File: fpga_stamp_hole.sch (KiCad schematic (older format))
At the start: 0 parts

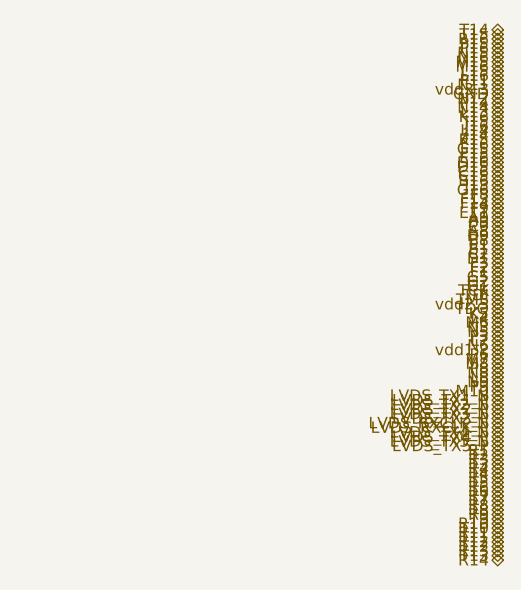
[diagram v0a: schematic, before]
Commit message: first commit
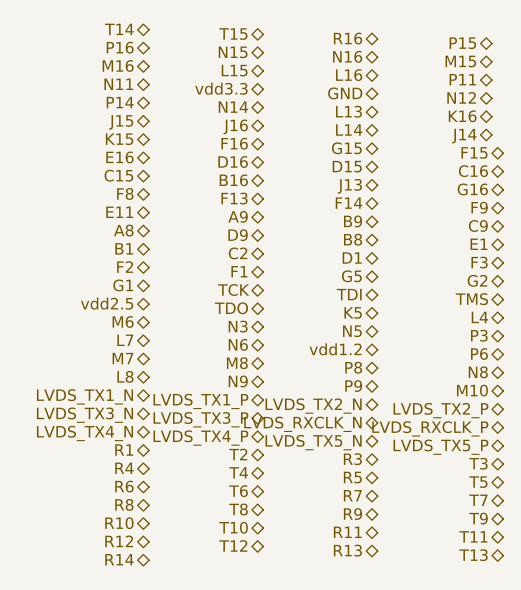
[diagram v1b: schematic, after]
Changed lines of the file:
@@
 $Descr A4 11693 8268
 encoding utf-8
-Sheet 2 2
+Sheet 2 3
 Title ""
 Date ""
@@
 EndData
 $EndBitmap
-Text HLabel 2550 1200 0    50   BiDi ~ 0
+Text HLabel 1000 1200 0    50   BiDi ~ 0
 T14
-Text HLabel 2550 1220 0    50   BiDi ~ 0
+Text HLabel 1500 1220 0    50   BiDi ~ 0
 T15
-Text HLabel 2550 1240 0    50   BiDi ~ 0
+Text HLabel 2000 1240 0    50   BiDi ~ 0
 R16
-Text HLabel 2550 1260 0    50   BiDi ~ 0
+Text HLabel 2500 1260 0    50   BiDi ~ 0
 P15
-Text HLabel 2550 1280 0    50   BiDi ~ 0
+Text HLabel 1000 1280 0    50   BiDi ~ 0
 P16
-Text HLabel 2550 1300 0    50   BiDi ~ 0
+Text HLabel 1500 1300 0    50   BiDi ~ 0
 N15
-Text HLabel 2550 1320 0    50   BiDi ~ 0
+Text HLabel 2000 1320 0    50   BiDi ~ 0
 N16
-Text HLabel 2550 1340 0    50   BiDi ~ 0
+Text HLabel 2500 1340 0    50   BiDi ~ 0
 M15
-Text HLabel 2550 1360 0    50   BiDi ~ 0
+Text HLabel 1000 1360 0    50   BiDi ~ 0
 M16
-Text HLabel 2550 1380 0    50   BiDi ~ 0
+Text HLabel 1500 1380 0    50   BiDi ~ 0
 L15
-Text HLabel 2550 1400 0    50   BiDi ~ 0
+Text HLabel 2000 1400 0    50   BiDi ~ 0
 L16
-Text HLabel 2550 1420 0    50   BiDi ~ 0
+Text HLabel 2500 1420 0    50   BiDi ~ 0
 P11
-Text HLabel 2550 1440 0    50   BiDi ~ 0
+Text HLabel 1000 1440 0    50   BiDi ~ 0
 N11
-Text HLabel 2550 1460 0    50   BiDi ~ 0
+Text HLabel 1500 1460 0    50   BiDi ~ 0
 vdd3.3
-Text HLabel 2550 1480 0    50   BiDi ~ 0
+Text HLabel 2000 1480 0    50   BiDi ~ 0
 GND
-Text HLabel 2550 1500 0    50   BiDi ~ 0
+Text HLabel 2500 1500 0    50   BiDi ~ 0
 N12
-Text HLabel 2550 1520 0    50   BiDi ~ 0
+Text HLabel 1000 1520 0    50   BiDi ~ 0
 P14
-Text HLabel 2550 1540 0    50   BiDi ~ 0
+Text HLabel 1500 1540 0    50   BiDi ~ 0
 N14
-Text HLabel 2550 1560 0    50   BiDi ~ 0
+Text HLabel 2000 1560 0    50   BiDi ~ 0
 L13
-Text HLabel 2550 1580 0    50   BiDi ~ 0
+Text HLabel 2500 1580 0    50   BiDi ~ 0
 K16
-Text HLabel 2550 1600 0    50   BiDi ~ 0
+Text HLabel 1000 1600 0    50   BiDi ~ 0
 J15
-Text HLabel 2550 1620 0    50   BiDi ~ 0
+Text HLabel 1500 1620 0    50   BiDi ~ 0
 J16
-Text HLabel 2550 1640 0    50   BiDi ~ 0
+Text HLabel 2000 1640 0    50   BiDi ~ 0
 L14
-Text HLabel 2550 1660 0    50   BiDi ~ 0
+Text HLabel 2500 1660 0    50   BiDi ~ 0
 J14
-Text HLabel 2550 1680 0    50   BiDi ~ 0
+Text HLabel 1000 1680 0    50   BiDi ~ 0
 K15
-Text HLabel 2550 1700 0    50   BiDi ~ 0
+Text HLabel 1500 1700 0    50   BiDi ~ 0
 F16
-Text HLabel 2550 1720 0    50   BiDi ~ 0
+Text HLabel 2000 1720 0    50   BiDi ~ 0
 G15
 Text HLabel 2550 1740 0    50   BiDi ~ 0
 F15
-Text HLabel 2550 1760 0    50   BiDi ~ 0
+Text HLabel 1000 1760 0    50   BiDi ~ 0
 E16
-Text HLabel 2550 1780 0    50   BiDi ~ 0
+Text HLabel 1500 1780 0    50   BiDi ~ 0
 D16
-Text HLabel 2550 1800 0    50   BiDi ~ 0
+Text HLabel 2000 1800 0    50   BiDi ~ 0
 D15
 Text HLabel 2550 1820 0    50   BiDi ~ 0
 C16
-Text HLabel 2550 1840 0    50   BiDi ~ 0
+Text HLabel 1000 1840 0    50   BiDi ~ 0
 C15
-Text HLabel 2550 1860 0    50   BiDi ~ 0
+Text HLabel 1500 1860 0    50   BiDi ~ 0
 B16
-Text HLabel 2550 1880 0    50   BiDi ~ 0
+Text HLabel 2000 1880 0    50   BiDi ~ 0
 J13
 Text HLabel 2550 1900 0    50   BiDi ~ 0
 G16
-Text HLabel 2550 1920 0    50   BiDi ~ 0
+Text HLabel 1000 1920 0    50   BiDi ~ 0
 F8
-Text HLabel 2550 1940 0    50   BiDi ~ 0
+Text HLabel 1500 1940 0    50   BiDi ~ 0
 F13
-Text HLabel 2550 1960 0    50   BiDi ~ 0
+Text HLabel 2000 1960 0    50   BiDi ~ 0
 F14
 Text HLabel 2550 1980 0    50   BiDi ~ 0
 F9
-Text HLabel 2550 2000 0    50   BiDi ~ 0
+Text HLabel 1000 2000 0    50   BiDi ~ 0
 E11
-Text HLabel 2550 2020 0    50   BiDi ~ 0
+Text HLabel 1500 2020 0    50   BiDi ~ 0
 A9
-Text HLabel 2550 2040 0    50   BiDi ~ 0
+Text HLabel 2000 2040 0    50   BiDi ~ 0
 B9
 Text HLabel 2550 2060 0    50   BiDi ~ 0
 C9
-Text HLabel 2550 2080 0    50   BiDi ~ 0
+Text HLabel 1000 2080 0    50   BiDi ~ 0
 A8
-Text HLabel 2550 2100 0    50   BiDi ~ 0
+Text HLabel 1500 2100 0    50   BiDi ~ 0
 D9
-Text HLabel 2550 2120 0    50   BiDi ~ 0
+Text HLabel 2000 2120 0    50   BiDi ~ 0
 B8
 Text HLabel 2550 2140 0    50   BiDi ~ 0
 E1
-Text HLabel 2550 2160 0    50   BiDi ~ 0
+Text HLabel 1000 2160 0    50   BiDi ~ 0
 B1
-Text HLabel 2550 2180 0    50   BiDi ~ 0
+Text HLabel 1500 2180 0    50   BiDi ~ 0
 C2
-Text HLabel 2550 2200 0    50   BiDi ~ 0
+Text HLabel 2000 2200 0    50   BiDi ~ 0
 D1
 Text HLabel 2550 2220 0    50   BiDi ~ 0
 F3
-Text HLabel 2550 2240 0    50   BiDi ~ 0
+Text HLabel 1000 2240 0    50   BiDi ~ 0
 F2
-Text HLabel 2550 2260 0    50   BiDi ~ 0
+Text HLabel 1500 2260 0    50   BiDi ~ 0
 F1
-Text HLabel 2550 2280 0    50   BiDi ~ 0
+Text HLabel 2000 2280 0    50   BiDi ~ 0
 G5
 Text HLabel 2550 2300 0    50   BiDi ~ 0
 G2
-Text HLabel 2550 2320 0    50   BiDi ~ 0
+Text HLabel 1000 2320 0    50   BiDi ~ 0
 G1
-Text HLabel 2550 2340 0    50   BiDi ~ 0
+Text HLabel 1500 2340 0    50   BiDi ~ 0
 TCK
-Text HLabel 2550 2360 0    50   BiDi ~ 0
+Text HLabel 2000 2360 0    50   BiDi ~ 0
 TDI
 Text HLabel 2550 2380 0    50   BiDi ~ 0
 TMS
-Text HLabel 2550 2400 0    50   BiDi ~ 0
+Text HLabel 1000 2400 0    50   BiDi ~ 0
 vdd2.5
-Text HLabel 2550 2420 0    50   BiDi ~ 0
+Text HLabel 1500 2420 0    50   BiDi ~ 0
 TDO
-Text HLabel 2550 2440 0    50   BiDi ~ 0
+Text HLabel 2000 2440 0    50   BiDi ~ 0
 K5
 Text HLabel 2550 2460 0    50   BiDi ~ 0
 L4
-Text HLabel 2550 2480 0    50   BiDi ~ 0
+Text HLabel 1000 2480 0    50   BiDi ~ 0
 M6
-Text HLabel 2550 2500 0    50   BiDi ~ 0
+Text HLabel 1500 2500 0    50   BiDi ~ 0
 N3
-Text HLabel 2550 2520 0    50   BiDi ~ 0
+Text HLabel 2000 2520 0    50   BiDi ~ 0
 N5
 Text HLabel 2550 2540 0    50   BiDi ~ 0
 P3
-Text HLabel 2550 2560 0    50   BiDi ~ 0
+Text HLabel 1000 2560 0    50   BiDi ~ 0
 L7
-Text HLabel 2550 2580 0    50   BiDi ~ 0
+Text HLabel 1500 2580 0    50   BiDi ~ 0
 N6
-Text HLabel 2550 2600 0    50   BiDi ~ 0
+Text HLabel 2000 2600 0    50   BiDi ~ 0
 vdd1.2
 Text HLabel 2550 2620 0    50   BiDi ~ 0
 P6
-Text HLabel 2550 2640 0    50   BiDi ~ 0
+Text HLabel 1000 2640 0    50   BiDi ~ 0
 M7
-Text HLabel 2550 2660 0    50   BiDi ~ 0
+Text HLabel 1500 2660 0    50   BiDi ~ 0
 M8
-Text HLabel 2550 2680 0    50   BiDi ~ 0
+Text HLabel 2000 2680 0    50   BiDi ~ 0
 P8
 Text HLabel 2550 2700 0    50   BiDi ~ 0
 N8
-Text HLabel 2550 2720 0    50   BiDi ~ 0
+Text HLabel 1000 2720 0    50   BiDi ~ 0
 L8
-Text HLabel 2550 2740 0    50   BiDi ~ 0
+Text HLabel 1500 2740 0    50   BiDi ~ 0
 N9
-Text HLabel 2550 2760 0    50   BiDi ~ 0
+Text HLabel 2000 2760 0    50   BiDi ~ 0
 P9
 Text HLabel 2550 2780 0    50   BiDi ~ 0
 M10
-Text HLabel 2550 2800 0    50   BiDi ~ 0
+Text HLabel 1000 2800 0    50   BiDi ~ 0
 LVDS_TX1_N
-Text HLabel 2550 2820 0    50   BiDi ~ 0
+Text HLabel 1500 2820 0    50   BiDi ~ 0
 LVDS_TX1_P
-Text HLabel 2550 2840 0    50   BiDi ~ 0
+Text HLabel 2000 2840 0    50   BiDi ~ 0
 LVDS_TX2_N
 Text HLabel 2550 2860 0    50   BiDi ~ 0
 LVDS_TX2_P
-Text HLabel 2550 2880 0    50   BiDi ~ 0
+Text HLabel 1000 2880 0    50   BiDi ~ 0
 LVDS_TX3_N
-Text HLabel 2550 2900 0    50   BiDi ~ 0
+Text HLabel 1500 2900 0    50   BiDi ~ 0
 LVDS_TX3_P
-Text HLabel 2550 2920 0    50   BiDi ~ 0
+Text HLabel 2000 2920 0    50   BiDi ~ 0
 LVDS_RXCLK_N
 Text HLabel 2550 2940 0    50   BiDi ~ 0
 LVDS_RXCLK_P
-Text HLabel 2550 2960 0    50   BiDi ~ 0
+Text HLabel 1000 2960 0    50   BiDi ~ 0
 LVDS_TX4_N
-Text HLabel 2550 2980 0    50   BiDi ~ 0
+Text HLabel 1500 2980 0    50   BiDi ~ 0
 LVDS_TX4_P
-Text HLabel 2550 3000 0    50   BiDi ~ 0
+Text HLabel 2000 3000 0    50   BiDi ~ 0
 LVDS_TX5_N
 Text HLabel 2550 3020 0    50   BiDi ~ 0
 LVDS_TX5_P
-Text HLabel 2550 3040 0    50   BiDi ~ 0
+Text HLabel 1000 3040 0    50   BiDi ~ 0
 R1
-Text HLabel 2550 3060 0    50   BiDi ~ 0
+Text HLabel 1500 3060 0    50   BiDi ~ 0
 T2
-Text HLabel 2550 3080 0    50   BiDi ~ 0
+Text HLabel 2000 3080 0    50   BiDi ~ 0
 R3
 Text HLabel 2550 3100 0    50   BiDi ~ 0
 T3
-Text HLabel 2550 3120 0    50   BiDi ~ 0
+Text HLabel 1000 3120 0    50   BiDi ~ 0
 R4
-Text HLabel 2550 3140 0    50   BiDi ~ 0
+Text HLabel 1500 3140 0    50   BiDi ~ 0
 T4
-Text HLabel 2550 3160 0    50   BiDi ~ 0
+Text HLabel 2000 3160 0    50   BiDi ~ 0
 R5
 Text HLabel 2550 3180 0    50   BiDi ~ 0
 T5
-Text HLabel 2550 3200 0    50   BiDi ~ 0
+Text HLabel 1000 3200 0    50   BiDi ~ 0
 R6
-Text HLabel 2550 3220 0    50   BiDi ~ 0
+Text HLabel 1500 3220 0    50   BiDi ~ 0
 T6
-Text HLabel 2550 3240 0    50   BiDi ~ 0
+Text HLabel 2000 3240 0    50   BiDi ~ 0
 R7
 Text HLabel 2550 3260 0    50   BiDi ~ 0
 T7
-Text HLabel 2550 3280 0    50   BiDi ~ 0
+Text HLabel 1000 3280 0    50   BiDi ~ 0
 R8
-Text HLabel 2550 3300 0    50   BiDi ~ 0
+Text HLabel 1500 3300 0    50   BiDi ~ 0
 T8
-Text HLabel 2550 3320 0    50   BiDi ~ 0
+Text HLabel 2000 3320 0    50   BiDi ~ 0
 R9
 Text HLabel 2550 3340 0    50   BiDi ~ 0
 T9
-Text HLabel 2550 3360 0    50   BiDi ~ 0
+Text HLabel 1000 3360 0    50   BiDi ~ 0
 R10
-Text HLabel 2550 3380 0    50   BiDi ~ 0
+Text HLabel 1500 3380 0    50   BiDi ~ 0
 T10
-Text HLabel 2550 3400 0    50   BiDi ~ 0
+Text HLabel 2000 3400 0    50   BiDi ~ 0
 R11
 Text HLabel 2550 3420 0    50   BiDi ~ 0
 T11
-Text HLabel 2550 3440 0    50   BiDi ~ 0
+Text HLabel 1000 3440 0    50   BiDi ~ 0
 R12
-Text HLabel 2550 3460 0    50   BiDi ~ 0
+Text HLabel 1500 3460 0    50   BiDi ~ 0
 T12
-Text HLabel 2550 3480 0    50   BiDi ~ 0
+Text HLabel 2000 3480 0    50   BiDi ~ 0
 R13
 Text HLabel 2550 3500 0    50   BiDi ~ 0
 T13
-Text HLabel 2550 3520 0    50   BiDi ~ 0
+Text HLabel 1000 3520 0    50   BiDi ~ 0
 R14
 $EndSCHEMATC
